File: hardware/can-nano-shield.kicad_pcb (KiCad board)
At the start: 2 copper layers, 18.1 x 43.6 mm, 24 parts, among them J1 Conn_01x15_Socket, J2 Conn_01x15_Socket, J3 Conn_01x04_Pin, J4 Conn_01x03_Socket, U1 MCP2515-xSO, U2 TJA1051T-3, Y1 16MHz 9pF

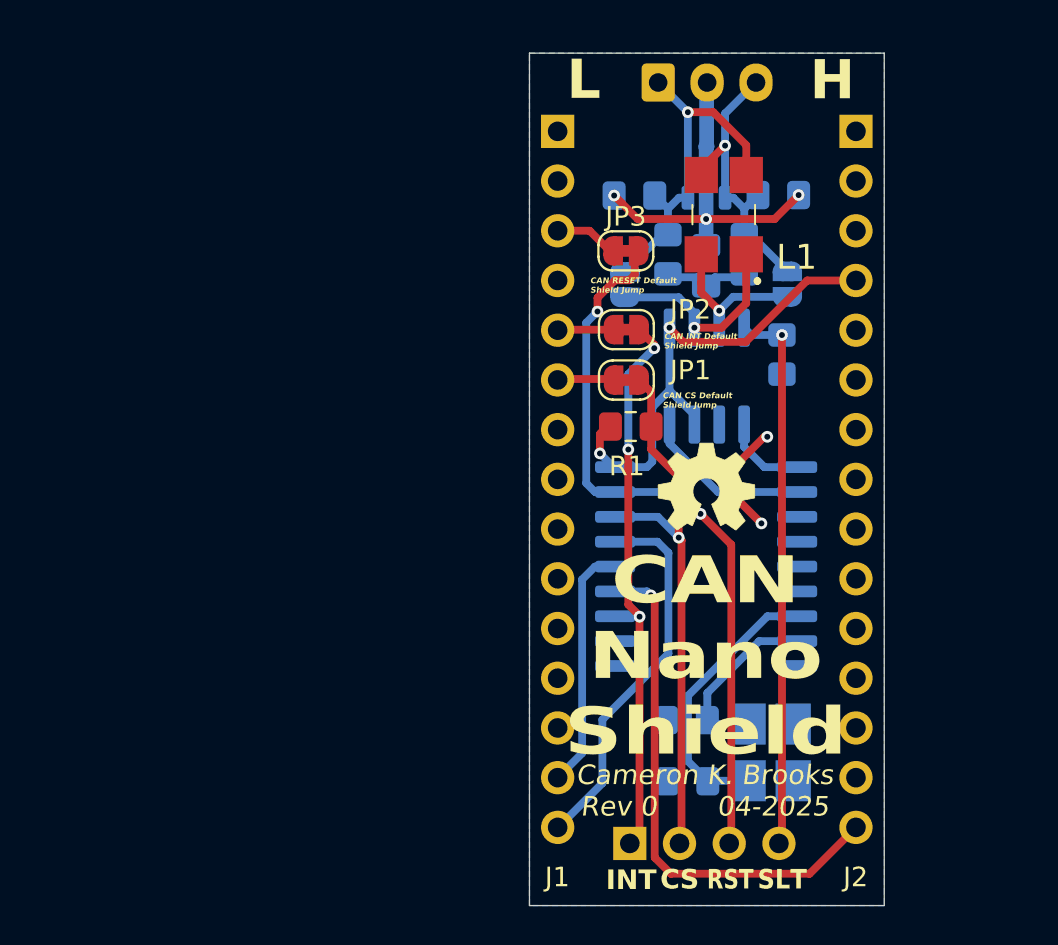
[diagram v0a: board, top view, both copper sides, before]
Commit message: added outputs
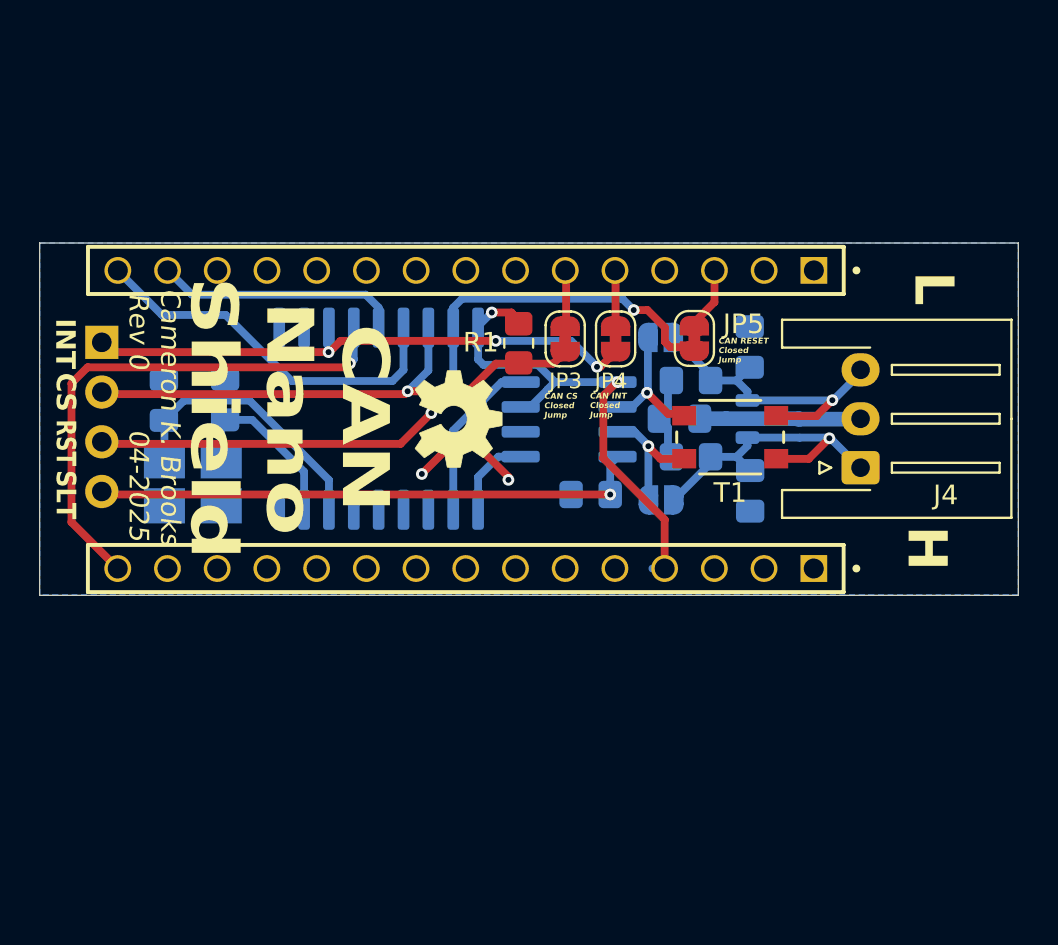
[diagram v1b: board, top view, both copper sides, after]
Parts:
- removed L1: B82789C0104N002, kml-custom:B82789C0113N002
- added T1: B82789C0113N002, kml-custom:SMT_13N002_TDK, F.Cu at (147.1, 93.2)
- J1, J2: value Conn_01x15_Socket -> SSQ-115-03-T-S; footprint Connector_PinHeader_2.54mm:PinHeader_1x15_P2.54mm_Vertical -> kml-custom:SAMTEC_SSQ-115-03-T-S; moved to F.Cu
- J4: moved to F.Cu
- R1: footprint Capacitor_SMD:C_0805_2012Metric_Pad1.18x1.45mm_HandSolder -> Resistor_SMD:R_0805_2012Metric_Pad1.20x1.40mm_HandSolder
- moved J3 37.2 mm to (115.0, 88.4), turned to 180 degrees
- moved C1 33.1 mm to (118.2, 91.3), turned to 90 degrees
- moved Y1 32.6 mm to (119.7, 95.6), turned to 0 degrees
- moved J2 29.9 mm to (133.6, 99.9)
- moved C2 28.7 mm to (121.3, 91.3), turned to 90 degrees
- moved J4 22.2 mm to (153.8, 94.8), turned to 90 degrees
- moved U1 18.4 mm to (129.2, 92.3), turned to 90 degrees
- moved C4 15.2 mm to (148.2, 96.0), turned to 90 degrees
- moved Ref** 13.4 mm to (133.0, 92.3), turned to -90 degrees
- moved D1 13.1 mm to (149.3, 92.3), turned to 0 degrees
- moved JP1 12.8 mm to (143.6, 96.4), turned to 0 degrees
- moved R2 12.1 mm to (140.0, 96.2), turned to 180 degrees
- moved Rt1 10.7 mm to (145.1, 94.2), turned to 180 degrees
- moved C5 9.72 mm to (148.1, 88.6), turned to 90 degrees
- moved J1 8.51 mm to (133.6, 84.7)
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- renumbered JP4 to JP1, JP5 to JP2, JP1 to JP3, JP2 to JP4, JP3 to JP5
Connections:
- J4 pad 1: /CAN_L -> /CAN_H
- J4 pad 3: /CAN_H -> /CAN_L
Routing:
- net GND: track 24.7 -> 14.1 mm, vias 6 -> 3
- net /CAN_L_IN: track 10.3 -> 7.32 mm
- net /CAN_L: track 18.2 -> 16.5 mm
- net /CAN_H: track 15.1 -> 16.4 mm
- net /CAN_H_IN: track 7.90 -> 7.09 mm
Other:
- board size 18.1 x 43.6 mm -> 50 x 18 mm
- board text added: "CAN CS Closed Jump"
- board text added: "CAN INT Closed Jump"
- board text added: "CAN RESET Closed Jump"
- board text removed: "CAN CS Default Shield Jump"
- board text removed: "CAN INT Default Shield Jump"
- board text removed: "CAN RESET Default Shield Jump"
